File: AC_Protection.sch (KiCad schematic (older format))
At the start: 1 part

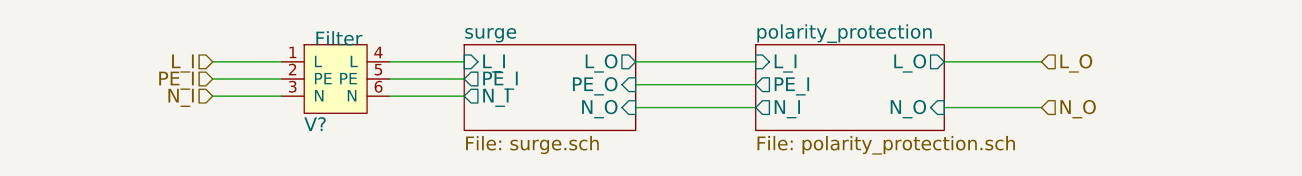
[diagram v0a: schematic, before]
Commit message: blub
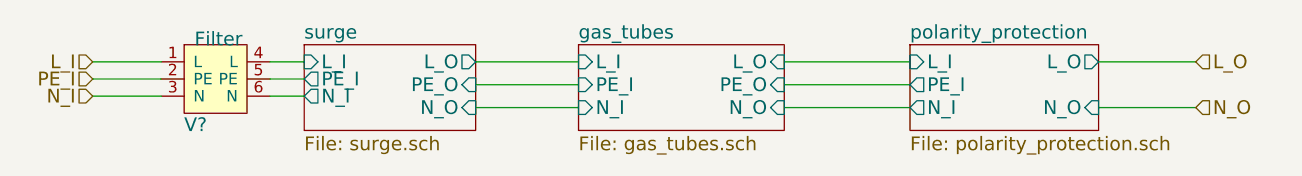
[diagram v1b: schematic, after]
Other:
- moved on the sheet: V?
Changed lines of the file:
@@
 $Descr A4 8268 11693 portrait
 encoding utf-8
-Sheet 7 12
+Sheet 5 13
 Title ""
 Date ""
@@
 $EndDescr
 $Sheet
-S 3050 4275 750  375
+S 2350 4275 750  375
 U 58B266CF
 F0 "surge" 60
 F1 "surge.sch" 60
-F2 "L_I" I L 3050 4350 60
-F3 "PE_I" O L 3050 4425 60
-F4 "N_I" O L 3050 4500 60
-F5 "L_O" O R 3800 4350 60
-F6 "PE_O" I R 3800 4450 60
-F7 "N_O" I R 3800 4550 60
+F2 "L_I" I L 2350 4350 60
+F3 "PE_I" O L 2350 4425 60
+F4 "N_I" O L 2350 4500 60
+F5 "L_O" O R 3100 4350 60
+F6 "PE_O" I R 3100 4450 60
+F7 "N_O" I R 3100 4550 60
 $EndSheet
-Text HLabel 1950 4350 0    60   Input ~ 0
+Text HLabel 1425 4350 0    60   Input ~ 0
 L_I
-Text HLabel 1950 4425 0    60   Input ~ 0
+Text HLabel 1425 4425 0    60   Input ~ 0
 PE_I
-Text HLabel 1950 4500 0    60   Input ~ 0
+Text HLabel 1425 4500 0    60   Input ~ 0
 N_I
-Text HLabel 5575 4350 2    60   Input ~ 0
+Text HLabel 6250 4350 2    60   Input ~ 0
 L_O
-Text HLabel 5575 4550 2    60   Input ~ 0
+Text HLabel 6250 4550 2    60   Input ~ 0
 N_O
 Wire Wire Line
-	1950 4350 2250 4350
+	1425 4350 1725 4350
 Wire Wire Line
-	2250 4425 1950 4425
+	1725 4425 1425 4425
 $Comp
 L Filter V?
 U 1 1 58B28B2C
-P 2500 4400
+P 1975 4400
 AR Path="/58B265C8/58B28B2C" Ref="V?"  Part="1"
 AR Path="/58B9DD1B/58BA5066/58B28B2C" Ref="V?"  Part="1"
-F 0 "V?" H 2400 4175 60  0000 C CNN
-F 1 "Filter" H 2500 4550 60  0000 C CNN
-F 2 "" H 2500 4400 60  0001 C CNN
-F 3 "" H 2500 4400 60  0001 C CNN
-	1    2500 4400
+F 0 "V?" H 1875 4175 60  0000 C CNN
+F 1 "Filter" H 1975 4550 60  0000 C CNN
+F 2 "" H 1975 4400 60  0001 C CNN
+F 3 "" H 1975 4400 60  0001 C CNN
+	1    1975 4400
 	1    0    0    -1
 $EndComp
 Wire Wire Line
-	2250 4500 1950 4500
+	1725 4500 1425 4500
 Wire Wire Line
-	2725 4350 3050 4350
+	2200 4350 2350 4350
 Wire Wire Line
-	2725 4425 3050 4425
+	2200 4425 2350 4425
 Wire Wire Line
-	2725 4500 3050 4500
+	2200 4500 2350 4500
 $Sheet
-S 4325 4275 825  375
+S 5000 4275 825  375
 U 58B2B6C6
 F0 "polarity_protection" 60
 F1 "polarity_protection.sch" 60
-F2 "L_I" I L 4325 4350 60
-F3 "PE_I" O L 4325 4450 60
-F4 "N_I" O L 4325 4550 60
-F5 "L_O" O R 5150 4350 60
-F6 "N_O" I R 5150 4550 60
+F2 "L_I" I L 5000 4350 60
+F3 "PE_I" O L 5000 4450 60
+F4 "N_I" O L 5000 4550 60
+F5 "L_O" O R 5825 4350 60
+F6 "N_O" I R 5825 4550 60
 $EndSheet
 Wire Wire Line
-	3800 4350 4325 4350
+	5825 4350 6250 4350
 Wire Wire Line
-	3800 4450 4325 4450
+	5825 4550 6250 4550
+$Sheet
+S 3550 4275 900  375
+U 58B67FE8
+F0 "gas_tubes" 60
+F1 "gas_tubes.sch" 60
+F2 "L_I" I L 3550 4350 60
+F3 "N_I" I L 3550 4550 60
+F4 "PE_I" I L 3550 4450 60
+F5 "L_O" I R 4450 4350 60
+F6 "N_O" I R 4450 4550 60
+F7 "PE_O" I R 4450 4450 60
+$EndSheet
 Wire Wire Line
-	3800 4550 4325 4550
+	3100 4350 3550 4350
 Wire Wire Line
-	5150 4350 5575 4350
+	3550 4450 3100 4450
 Wire Wire Line
-	5150 4550 5575 4550
+	3100 4550 3550 4550
+Wire Wire Line
+	4450 4550 5000 4550
+Wire Wire Line
+	5000 4450 4450 4450
+Wire Wire Line
+	4450 4350 5000 4350
 $EndSCHEMATC
